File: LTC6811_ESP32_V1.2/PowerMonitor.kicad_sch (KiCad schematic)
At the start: 51 parts, among them U2 AMC1301 or AMC1302, U3 AMC1301, U5 OPA2197IDR, U6 ISL28022

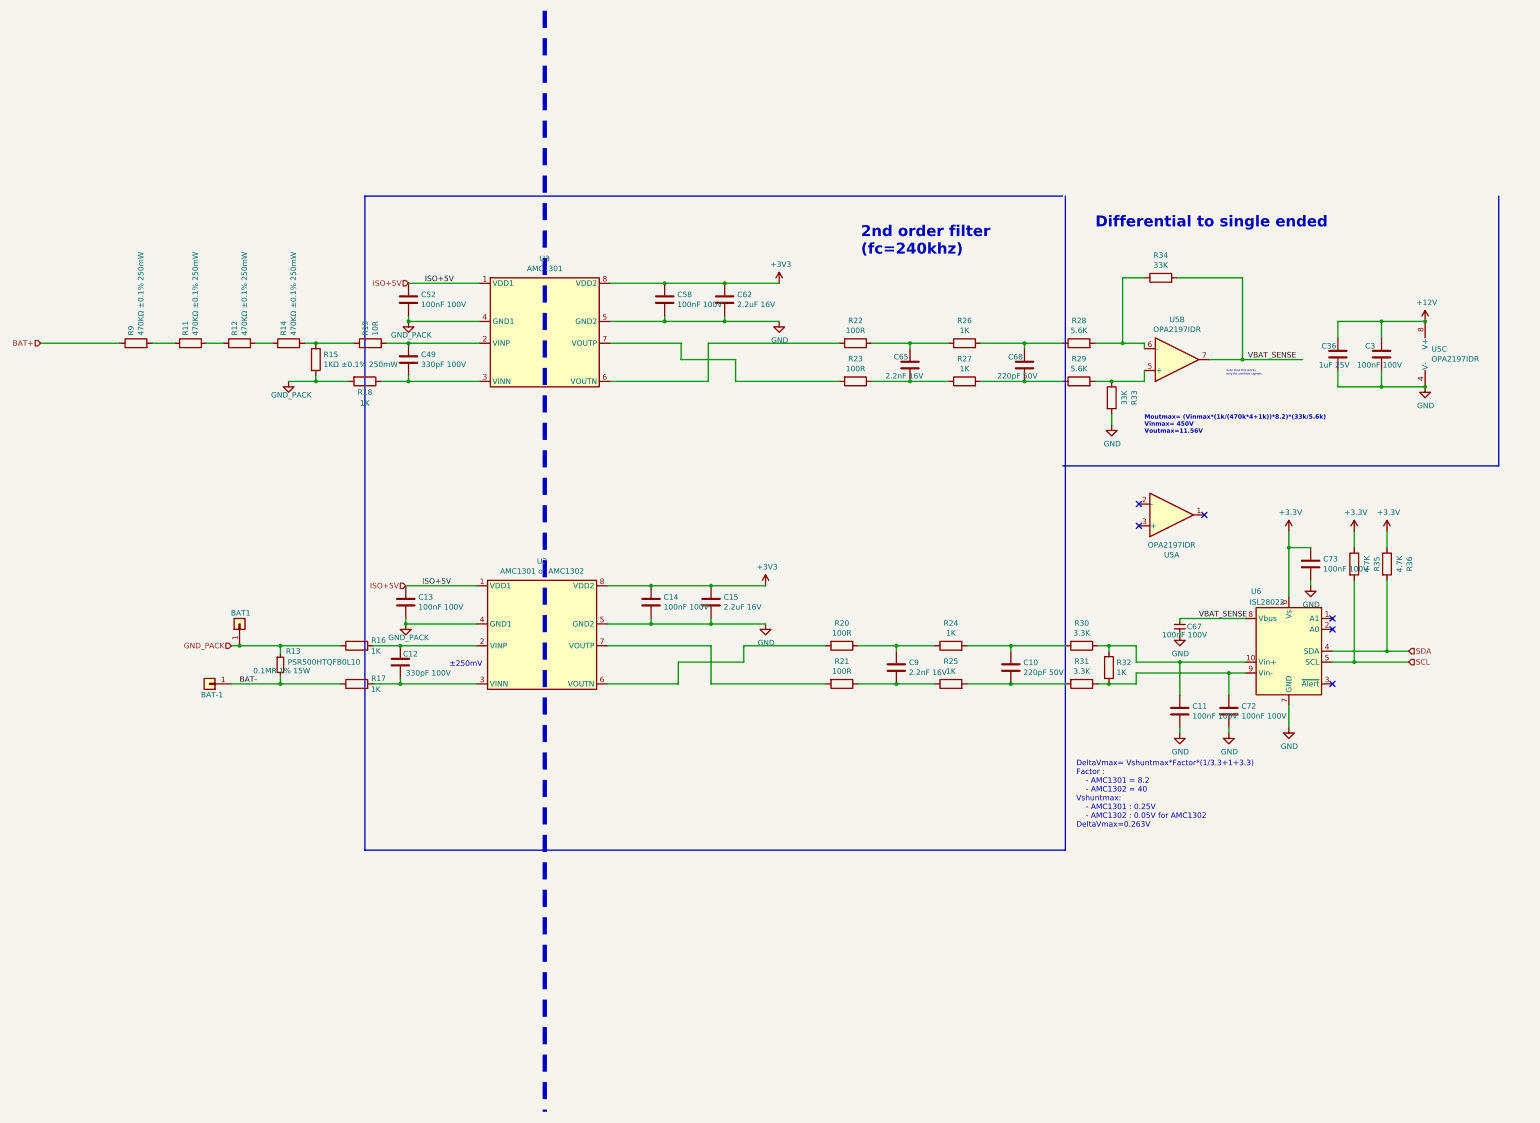
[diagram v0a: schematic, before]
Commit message: Add files via upload
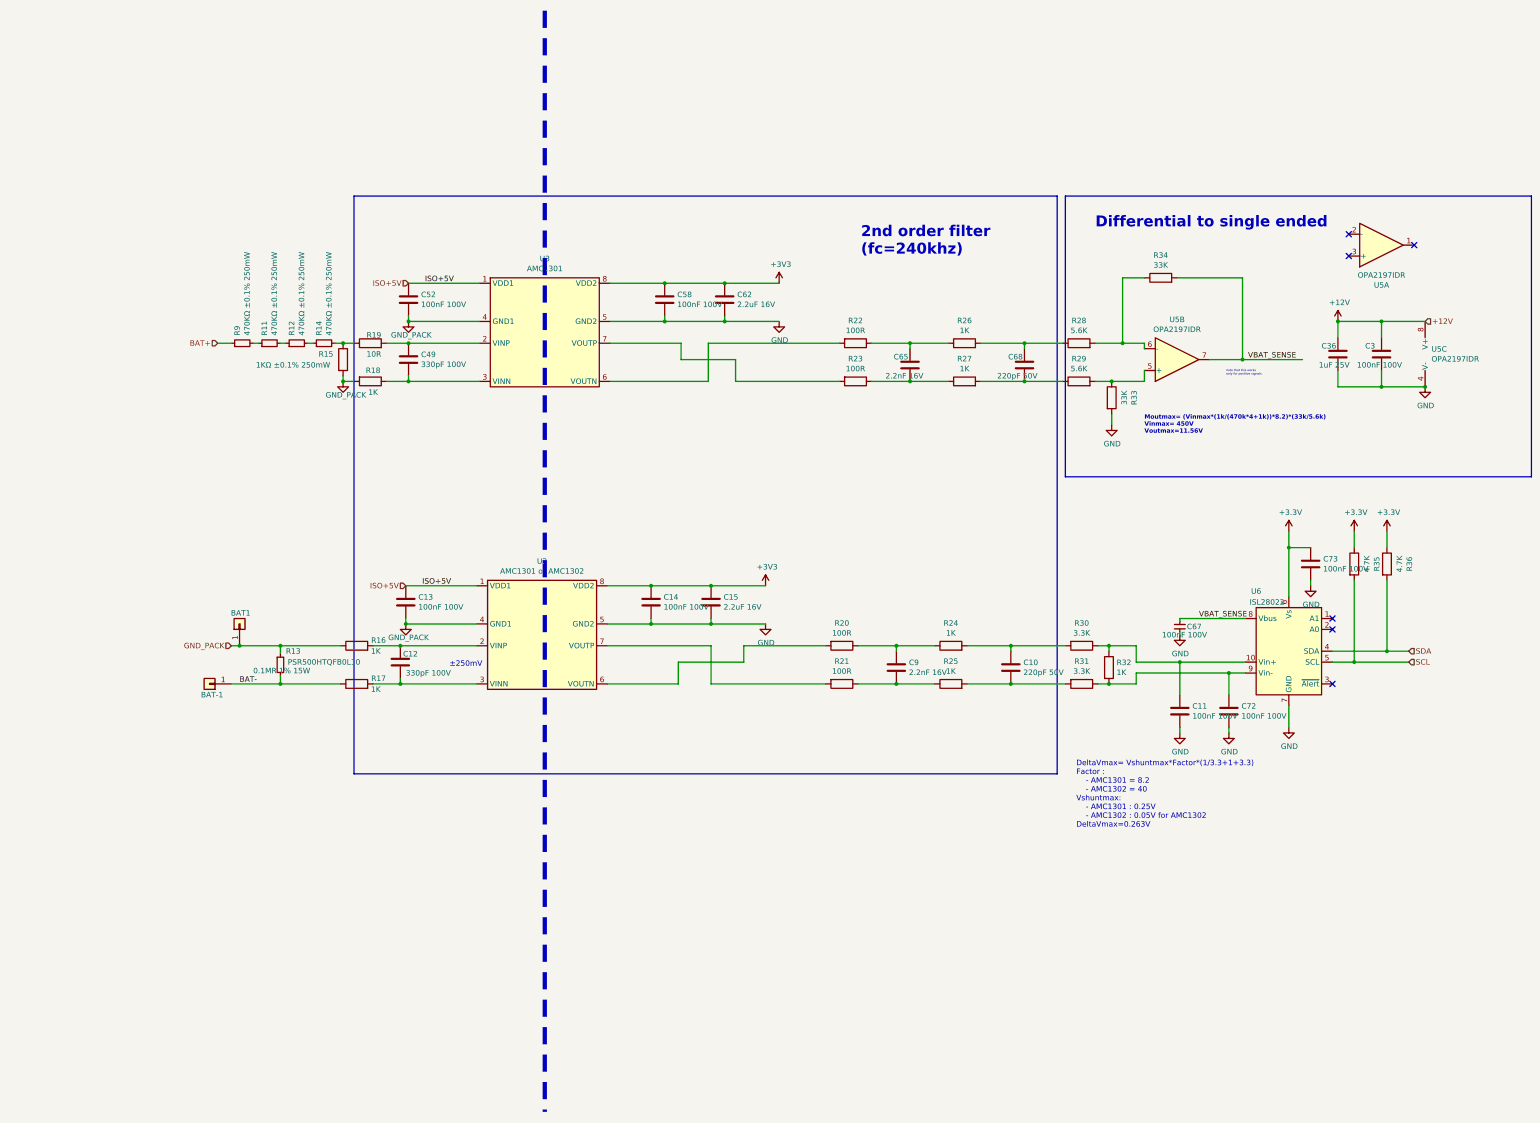
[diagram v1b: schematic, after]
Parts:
- R11, R12, R14, R9: symbol BMS-Master-rescue:R-Device-BMS-Master-rescue -> Device:R_Small
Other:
- moved on the sheet: R11, R12, R14, R15, R18, R9, U5A
